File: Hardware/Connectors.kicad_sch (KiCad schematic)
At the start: 27 parts, among them J1 Conn_01x03, J2 Conn_01x07, SW9 SW_Push

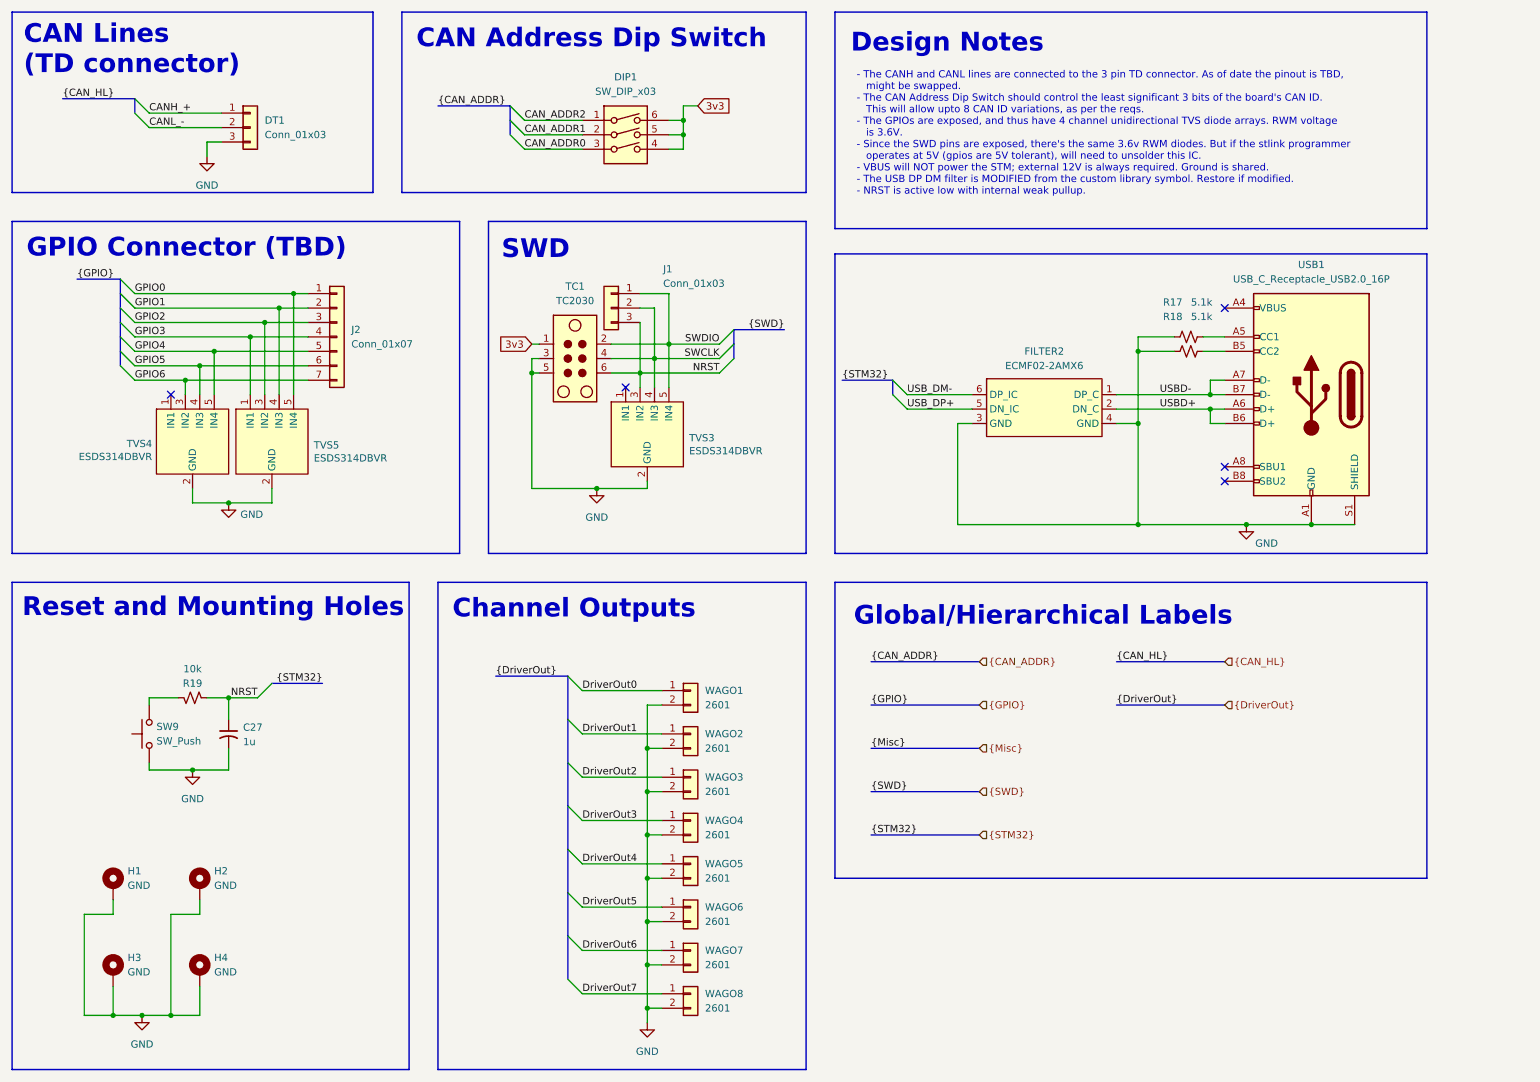
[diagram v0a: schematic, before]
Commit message: temp
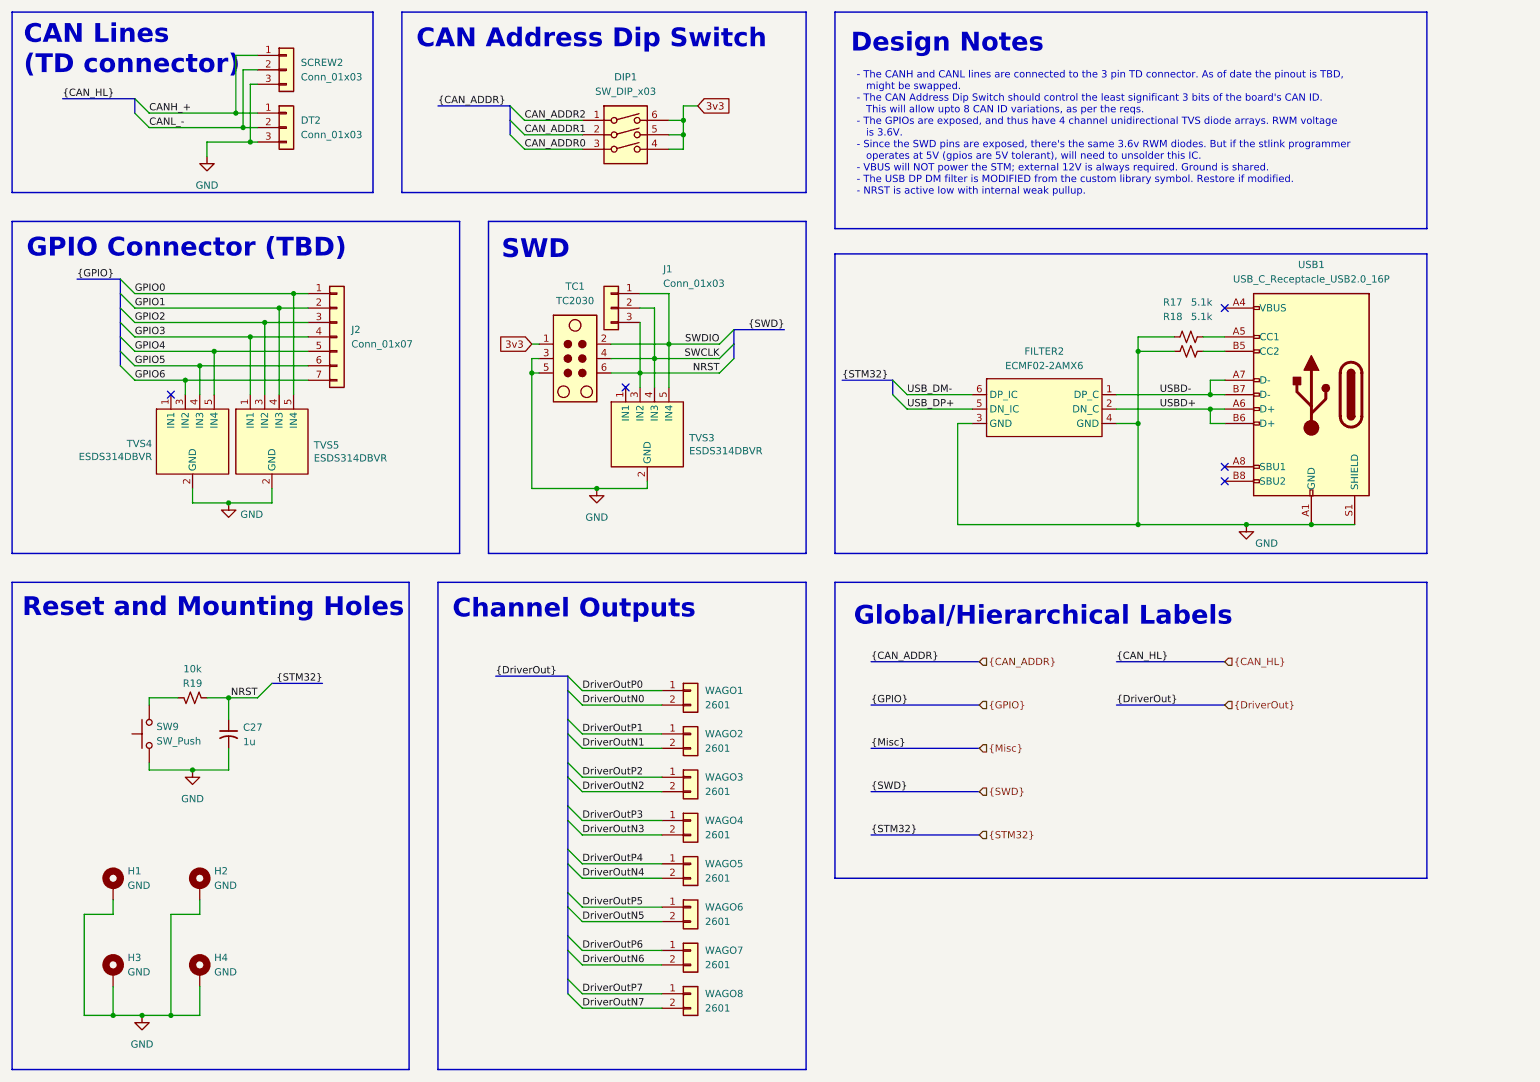
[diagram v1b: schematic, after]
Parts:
- added SCREW2: Conn_01x03, TerminalBlock:TerminalBlock_MaiXu_MX126-5.0-03P_1x03_P5.00mm, symbol Connector_Generic:Conn_01x03
- DT2: renamed from DT1; footprint TerminalBlock:TerminalBlock_MaiXu_MX126-5.0-03P_1x03_P5.00mm -> footprints:TE_DTF13-3P
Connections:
- net CANH_+: now also SCREW2.1 (Pin_1)
- net CANL_-: now also SCREW2.2 (Pin_2)
- net GND: now also SCREW2.3 (Pin_3); no longer WAGO1.2 (Pin_2), WAGO2.2 (Pin_2), WAGO3.2 (Pin_2), WAGO4.2 (Pin_2), WAGO5.2 (Pin_2), WAGO6.2 (Pin_2), WAGO7.2 (Pin_2), WAGO8.2 (Pin_2)
- net DriverOut0 renamed DriverOutP0
- net DriverOut1 renamed DriverOutP1
- net DriverOut2 renamed DriverOutP2
- net DriverOut3 renamed DriverOutP3
- net DriverOut4 renamed DriverOutP4
- net DriverOut5 renamed DriverOutP5
- net DriverOut6 renamed DriverOutP6
- net DriverOut7 renamed DriverOutP7
- new net DriverOutN0: WAGO1.2 (Pin_2)
- new net DriverOutN1: WAGO2.2 (Pin_2)
- new net DriverOutN2: WAGO3.2 (Pin_2)
- new net DriverOutN3: WAGO4.2 (Pin_2)
- new net DriverOutN4: WAGO5.2 (Pin_2)
- new net DriverOutN5: WAGO6.2 (Pin_2)
- new net DriverOutN6: WAGO7.2 (Pin_2)
- new net DriverOutN7: WAGO8.2 (Pin_2)
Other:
- moved on the sheet: DT2
